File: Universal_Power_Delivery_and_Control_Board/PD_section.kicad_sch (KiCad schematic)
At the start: 74 parts, among them Q1 PMZ600UNEYL, Q2 PMZ600UNEYL, U1 TPS259470LRPWR, U18 LM66200DRLR, U2 CH224Q_C46061833, U21 TPS22919DCK, U3 USBLC6-2SC6, U4 ESD2CAN24-ES, U5 S2B-ZR (LF)(SN), U6 USBLC6-2SC6, U7 TPS54202DDC

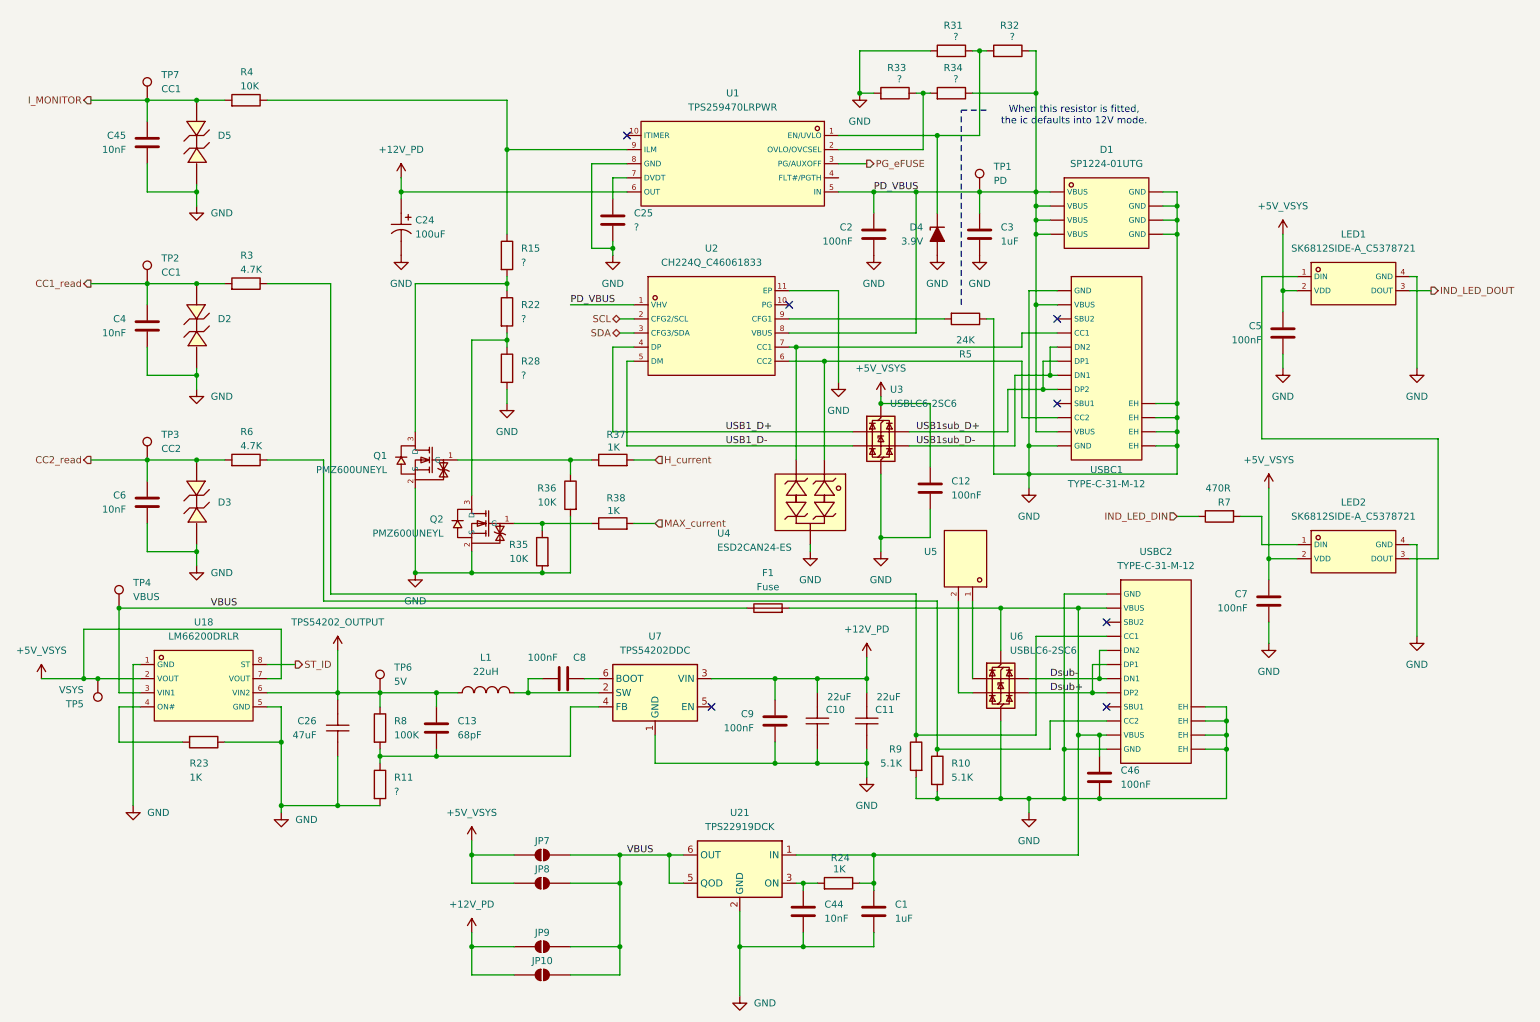
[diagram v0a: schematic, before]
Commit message: Fished layout for now, need to add some components for optional functionality.
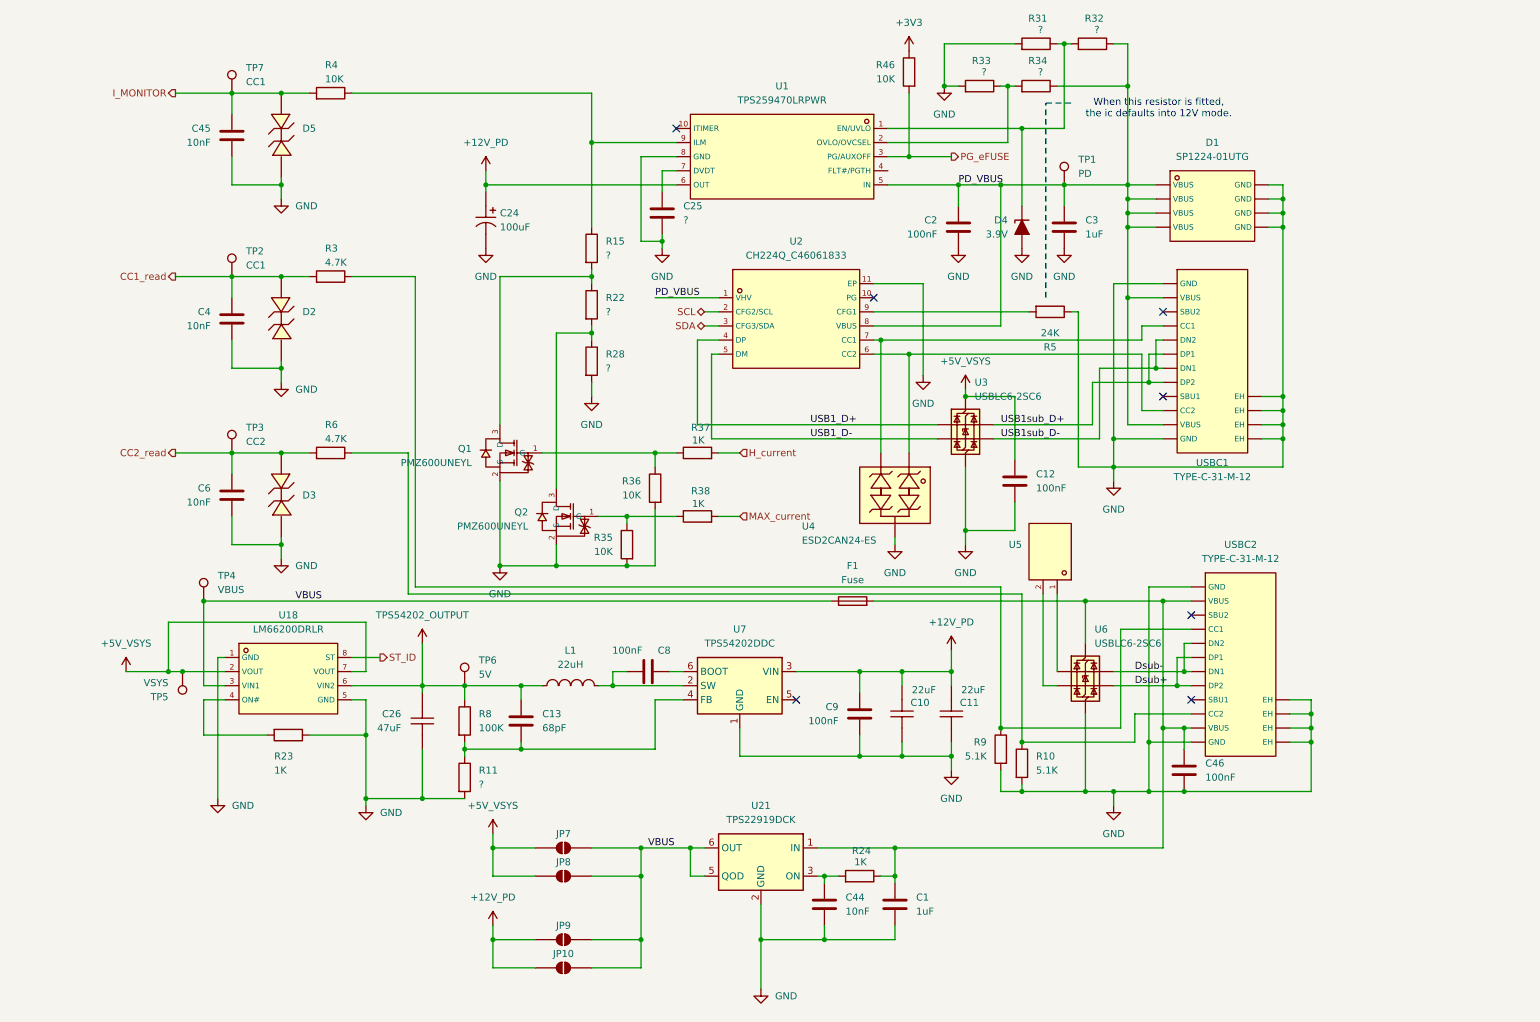
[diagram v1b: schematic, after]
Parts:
- removed C5, C7: 100nF, Capacitor_SMD:C_0402_1005Metric_Pad0.74x0.62mm_HandSolder, symbol Device:C
- removed LED1, LED2: SK6812SIDE-A_C5378721, lcsc_footprints:C5378721_LED-SMD_4P-L4_0-W1_6-L, symbol lcsc_imported:SK6812SIDE-A_C5378721
- removed R7: 470R, Resistor_SMD:R_0402_1005Metric_Pad0.72x0.64mm_HandSolder, symbol Device:R
- added R46: 10K, Resistor_SMD:R_0402_1005Metric_Pad0.72x0.64mm_HandSolder, symbol Device:R
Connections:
- net PG_eFUSE: now also R46.2
- new net +3V3: R46.1
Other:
- moved on the sheet: C1, C10, C11, C12, C13, C2, C24, C25, C26, C3, C4, C44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
